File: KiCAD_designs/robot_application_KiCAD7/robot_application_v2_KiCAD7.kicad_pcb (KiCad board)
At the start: 2 copper layers, 32.5 x 22.4 mm, 6 parts, among them J1 B2B-PH-SM4-TBT LFSN, J2 B2B-PH-SM4-TBT LFSN, Q1 AO3400A, U1 ATTINY85-20SUR

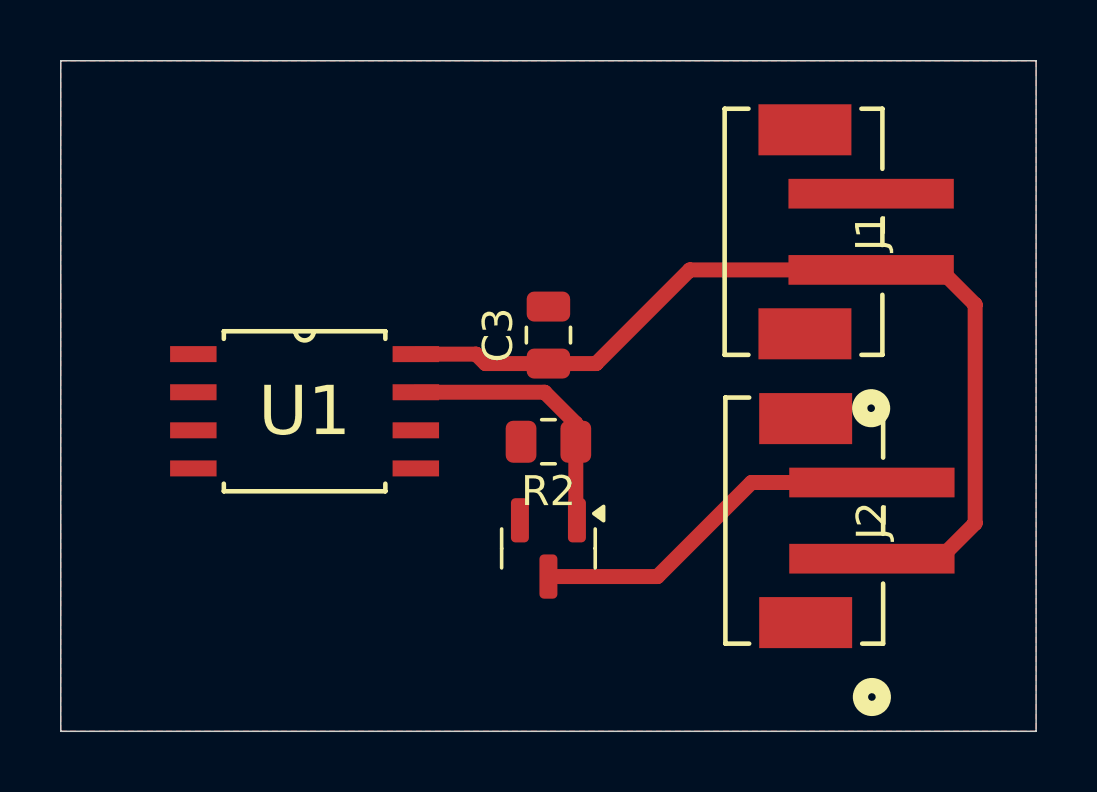
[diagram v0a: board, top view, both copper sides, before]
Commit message: esp v1
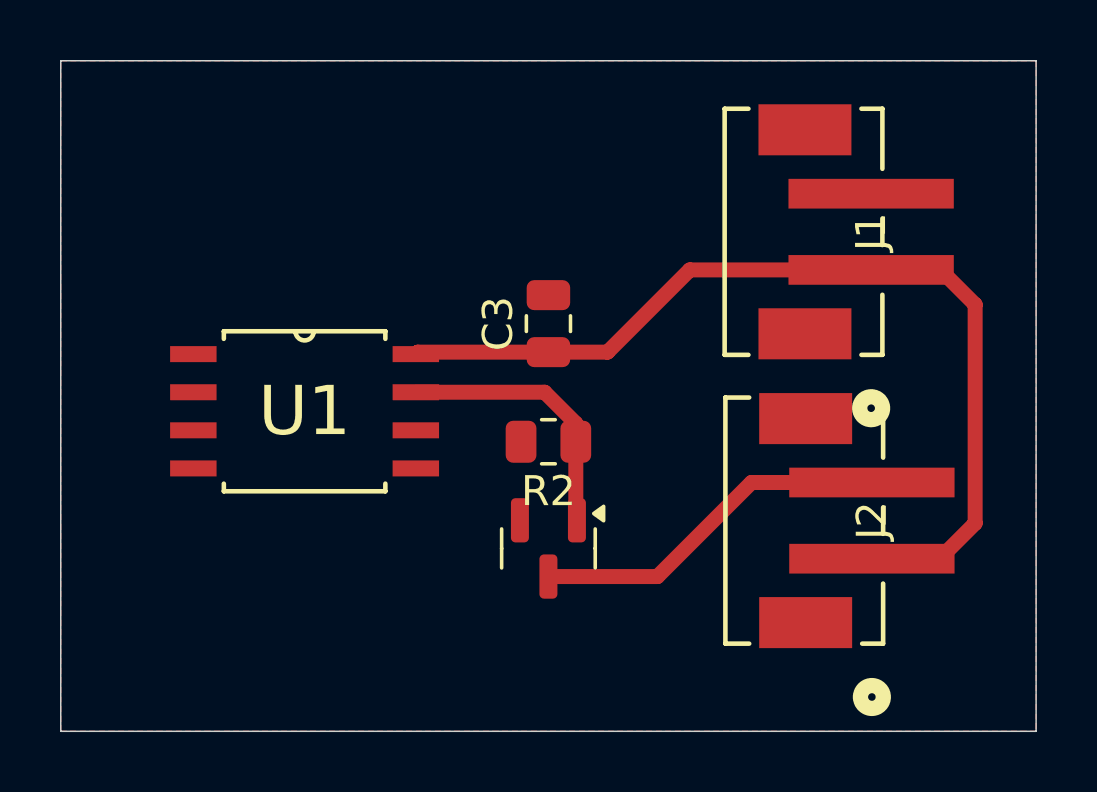
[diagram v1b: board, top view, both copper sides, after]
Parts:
- moved C3 0.38 mm to (43.2, 30.6)
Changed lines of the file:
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@@
     (pad_to_mask_clearance 0)
     (pcbplotparams
-      (layerselection 0x00010fc_ffffffff)
+      (layerselection 0x0001000_7fffffff)
       (plot_on_all_layers_selection 0x0000000_00000000)
       (disableapertmacros false)
@@
       (outputformat 1)
       (mirror false)
-      (drillshape 1)
+      (drillshape 0)
       (scaleselection 1)
       (outputdirectory "")
@@
     (fp_line (start 1 0.625) (end -1 0.625)
       (stroke (width 0.1) (type solid)) (layer "F.Fab"))
-    (pad "1" smd roundrect (at -0.9125 0 180) (size 1.025 1.4) (layers "F.Cu" "F.Paste" "F.Mask") (roundrect_rratio 0.243902)
+    (pad "1" smd roundrect (at -0.9125 0 180) (size 1.025 1.4) (layers "F.Cu" "F.Paste" "F.Mask") (roundrect_rratio 0.243902439)
       (net 4 "/signal") (pintype "passive"))
-    (pad "2" smd roundrect (at 0.9125 0 180) (size 1.025 1.4) (layers "F.Cu" "F.Paste" "F.Mask") (roundrect_rratio 0.243902)
+    (pad "2" smd roundrect (at 0.9125 0 180) (size 1.025 1.4) (layers "F.Cu" "F.Paste" "F.Mask") (roundrect_rratio 0.243902439)
       (net 1 "GND") (pintype "passive"))
     (model "${KICAD6_3DMODEL_DIR}/Resistor_SMD.3dshapes/R_0805_2012Metric.wrl"
@@
   )
   (footprint "Capacitor_SMD:C_0805_2012Metric" (layer "F.Cu")
-    (at 43.18 30.988 90)
+    (at 43.18 30.607 90)
     (descr "Capacitor SMD 0805 (2012 Metric), square (rectangular) end terminal, IPC_7351 nominal, (Body size source: IPC-SM-782 page 76, https://www.pcb-3d.com/wordpress/wp-content/uploads/ipc-sm-782a_amendment_1_and_2.pdf, https://docs.google.com/spreadsheets/d/1BsfQQcO9C6DZCsRaXUlFlo91Tg2WpOkGARC1WS5S8t0/edit?usp=sharing), generated with kicad-footprint-generator")
     (tags "capacitor")
@@
   (gr_rect (start 26.924 21.844) (end 59.436 44.196)
     (stroke (width 0.05) (type default)) (fill none) (layer "Edge.Cuts"))
+  (segment (start 43.18 31.557) (end 38.8264 31.557) (width 0.5) (layer "F.Cu") (net 3))
   (segment (start 53.961866 38.442408) (end 56.222466 38.442408) (width 0.5) (layer "F.Cu") (net 3))
   (segment (start 57.404 29.972) (end 56.247818 28.815818) (width 0.5) (layer "F.Cu") (net 3))
   (segment (start 57.404 37.260874) (end 57.404 29.972) (width 0.5) (layer "F.Cu") (net 3))
+  (segment (start 45.151 31.557) (end 43.18 31.557) (width 0.5) (layer "F.Cu") (net 3))
   (segment (start 56.247818 28.815818) (end 53.937247 28.815818) (width 0.5) (layer "F.Cu") (net 3))
-  (segment (start 44.77 31.938) (end 47.892182 28.815818) (width 0.5) (layer "F.Cu") (net 3))
-  (segment (start 41.082 31.938) (end 40.767 31.623) (width 0.5) (layer "F.Cu") (net 3))
   (segment (start 47.892182 28.815818) (end 53.937247 28.815818) (width 0.5) (layer "F.Cu") (net 3))
-  (segment (start 43.18 31.938) (end 41.082 31.938) (width 0.5) (layer "F.Cu") (net 3))
-  (segment (start 40.767 31.623) (end 38.7604 31.623) (width 0.5) (layer "F.Cu") (net 3))
+  (segment (start 38.8264 31.557) (end 38.7604 31.623) (width 0.5) (layer "F.Cu") (net 3))
+  (segment (start 47.892182 28.815818) (end 45.151 31.557) (width 0.5) (layer "F.Cu") (net 3))
   (segment (start 56.222466 38.442408) (end 57.404 37.260874) (width 0.5) (layer "F.Cu") (net 3))
-  (segment (start 43.18 31.938) (end 44.77 31.938) (width 0.5) (layer "F.Cu") (net 3))
   (segment (start 44.0925 37.125) (end 44.13 37.1625) (width 0.5) (layer "F.Cu") (net 4))
   (segment (start 43.053 32.893) (end 44.0925 33.9325) (width 0.5) (layer "F.Cu") (net 4))
